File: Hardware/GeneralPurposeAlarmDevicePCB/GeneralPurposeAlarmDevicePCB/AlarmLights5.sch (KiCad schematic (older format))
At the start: 20 parts, among them Q201 MMBT2222A-7-F, Q202 MMBT2222A-7-F, Q203 MMBT2222A-7-F, Q204 MMBT2222A-7-F, Q205 MMBT2222A-7-F

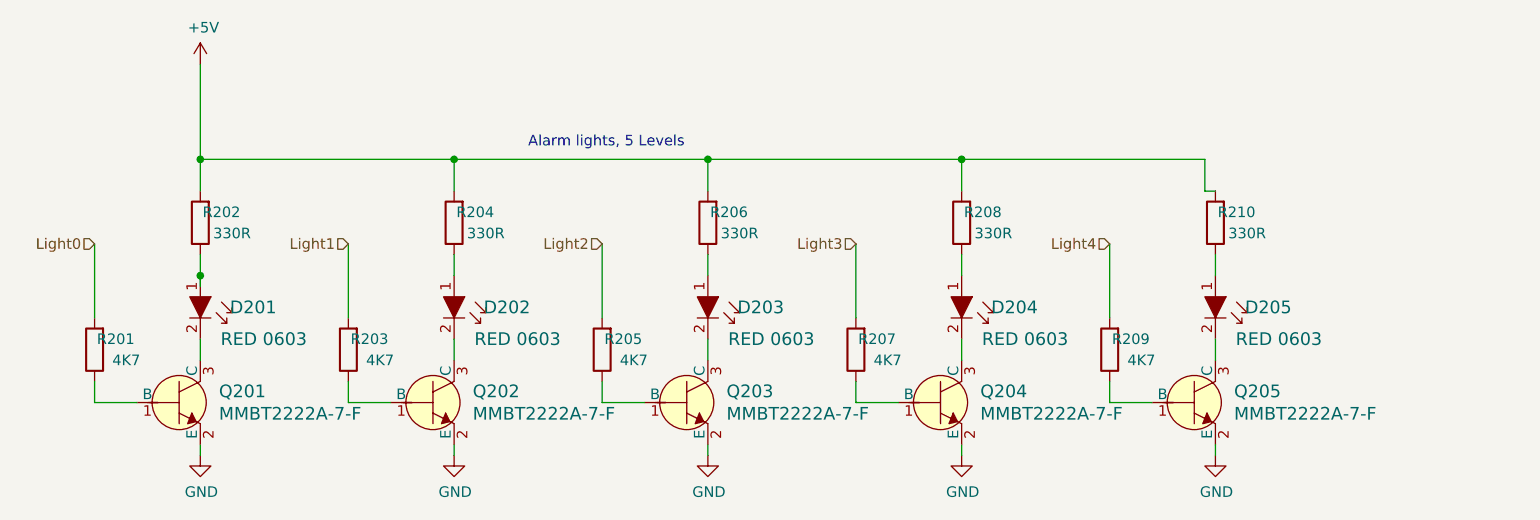
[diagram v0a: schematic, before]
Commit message: Add new LED, RJ12 footprints to footprint library. Add STEP model.
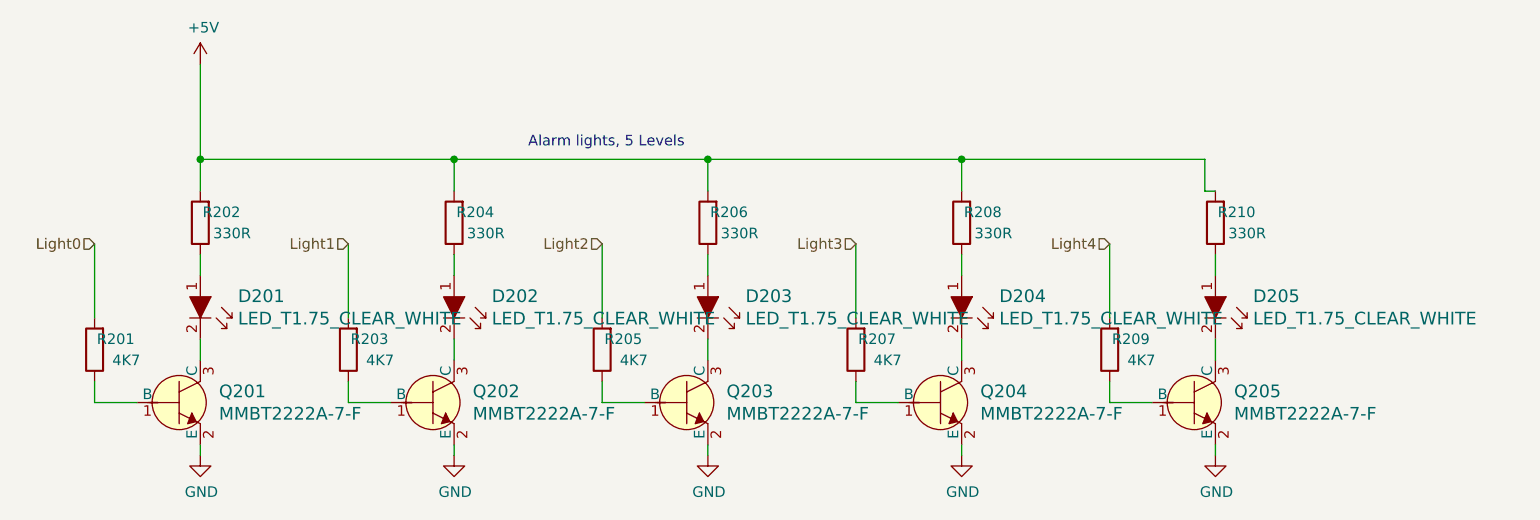
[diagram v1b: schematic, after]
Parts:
- removed D201, D202, D203, D204, D205: RED 0603, LED_SMD:LED_0603_1608Metric, symbol dk_LED-Indication-Discrete:LTST-C171KRKT
- added D201, D202, D203, D204, D205: LED_T1.75_CLEAR_WHITE, GeneralPurposeAlarmDevicePCB:LED_5mm_Radial, symbol GPAD_SCH_LIB:LED_T1.75_CLEAR_WHITE
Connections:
- net at R202.1: now also D201.1
- net at Q201.3 (C): now also D201.2
- net at R204.1: now also D202.1
- net at Q202.3 (C): now also D202.2
- net at R206.1: now also D203.1
- net at Q203.3 (C): now also D203.2
- net at R208.1: now also D204.1
- net at Q204.3 (C): now also D204.2
- net at R210.1: now also D205.1
- net at Q205.3 (C): now also D205.2

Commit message: Add JST connector for I2C and more.
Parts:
- removed Q201, Q202, Q203, Q204, Q205: MMBT2222A-7-F, digikey-footprints:SOT-23-3, symbol dk_Transistors-Bipolar-BJT-Single:MMBT2222A-7-F
- added Q201, Q202, Q203, Q204, Q205: MMBT2222A-7-F, Package_TO_SOT_SMD:SOT-23, symbol GPAD_SCH_LIB:MMBT2222A-7-F
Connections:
- net GND: now also Q201.2 (E), Q202.2 (E), Q203.2 (E), Q204.2 (E), Q205.2 (E)
- net at R201.1: now also Q201.1 (B)
- net at D201.2: now also Q201.3 (C)
- net at R203.1: now also Q202.1 (B)
- net at D202.2: now also Q202.3 (C)
- net at R205.1: now also Q203.1 (B)
- net at D203.2: now also Q203.3 (C)
- net at R207.1: now also Q204.1 (B)
- net at D204.2: now also Q204.3 (C)
- net at R209.1: now also Q205.1 (B)
- net at D205.2: now also Q205.3 (C)
